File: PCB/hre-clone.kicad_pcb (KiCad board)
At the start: 2 copper layers, 155.5 x 76.9 mm, 23 parts, among them SW1 SW_DIP_x04, U1 74LS258, U10 MC6845, U11 MC6845, U12 DIL14, U13 7402, U2 74LS174, U3 74LS257, U4 74LS244, U5 2716, U6 2716, U7 74LS05, U8 74LS155, U9 74LS257

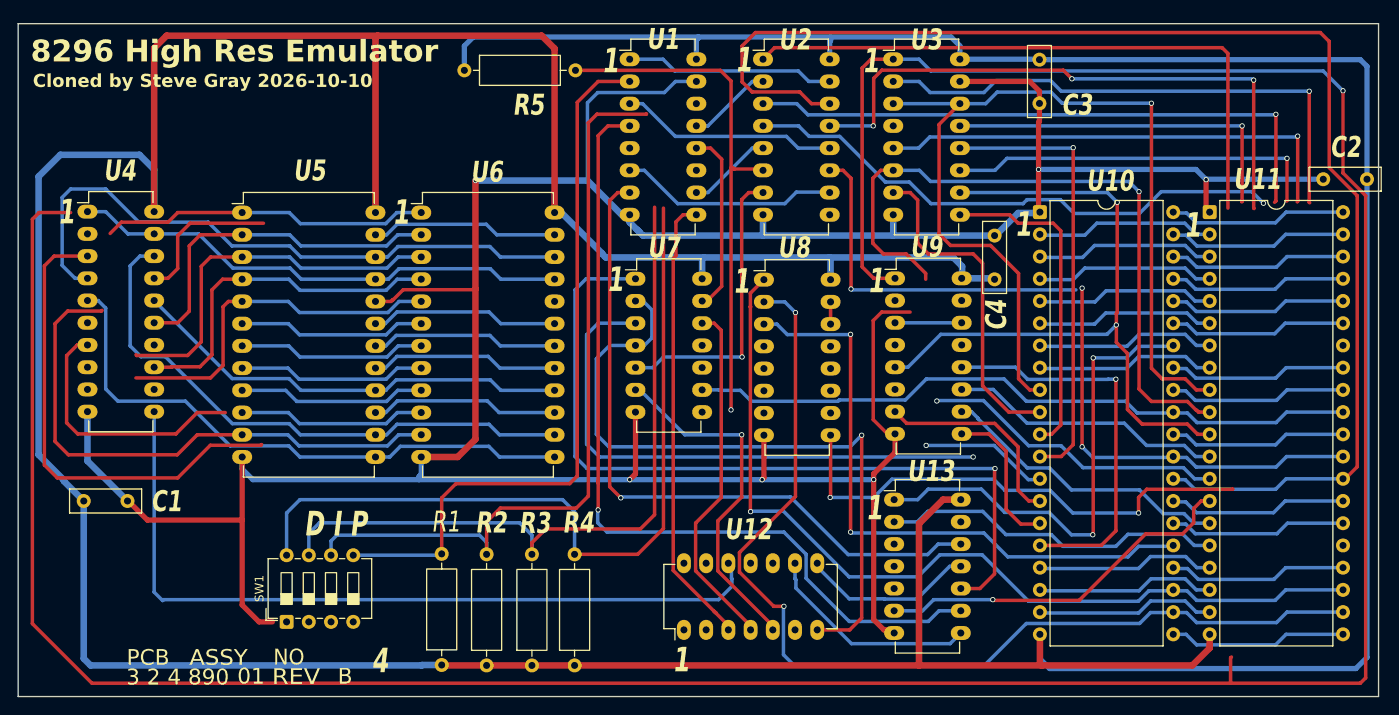
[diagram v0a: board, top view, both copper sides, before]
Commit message: Re-organize file, remove backup files, update readme
A little more organization always helps!
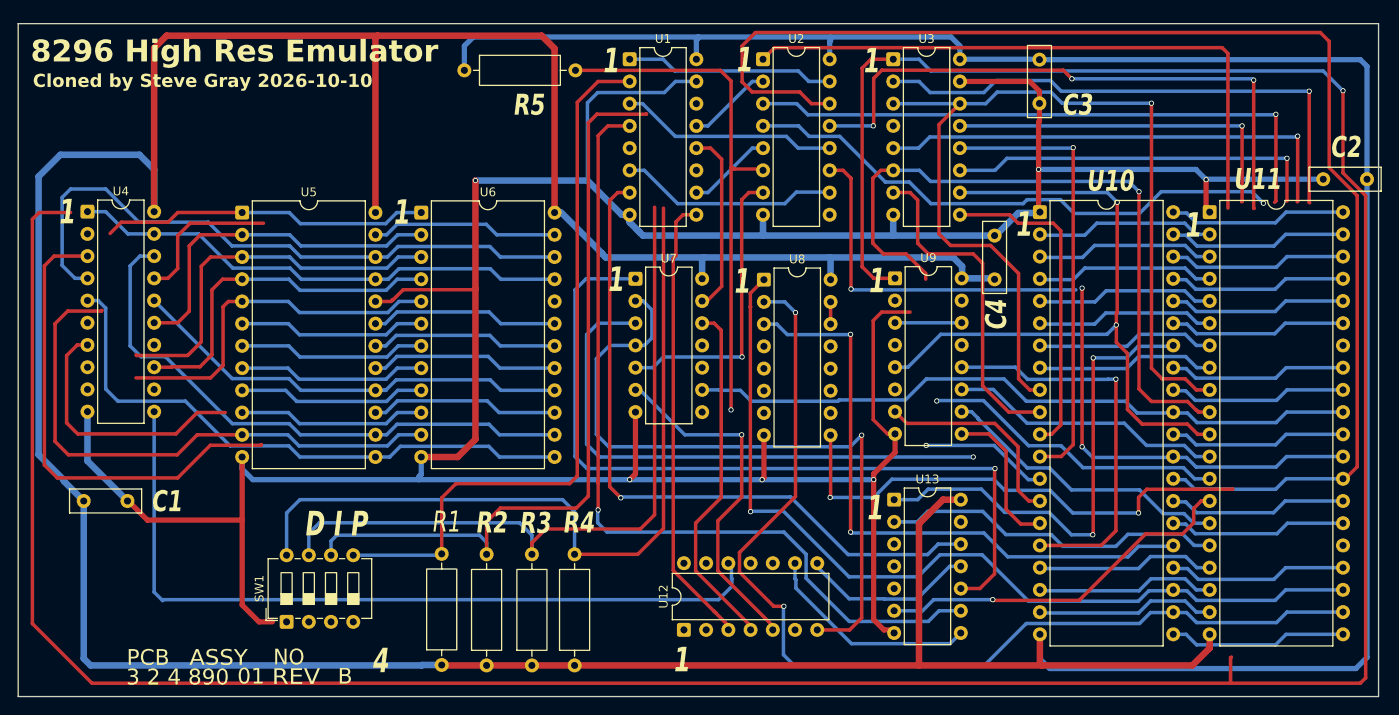
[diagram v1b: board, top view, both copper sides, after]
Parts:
- U1, U2, U3, U8, U9: footprint Housings_DIP:DIP-16_W7.62mm_LongPads -> Package_DIP:DIP-16_W7.62mm
- U12, U13, U7: footprint Housings_DIP:DIP-14_W7.62mm_LongPads -> Package_DIP:DIP-14_W7.62mm
- U4: footprint Housings_DIP:DIP-20_W7.62mm_LongPads -> Package_DIP:DIP-20_W7.62mm
- U5, U6: footprint Housings_DIP:DIP-24_W15.24mm_LongPads -> Package_DIP:DIP-24_W15.24mm
